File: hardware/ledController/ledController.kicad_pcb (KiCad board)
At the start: 2 copper layers, 50 x 50 mm, 33 parts, among them IC1 PIC16F1769-I_ML, J1 Conn_01x06, J2 Screw_Terminal_01x02, J3 Screw_Terminal_01x02, J4 Conn_01x06, J5 Conn_01x02_Male, M1 LM2596_module, Q1 FMMT458TA, Q2 BUJ302AD

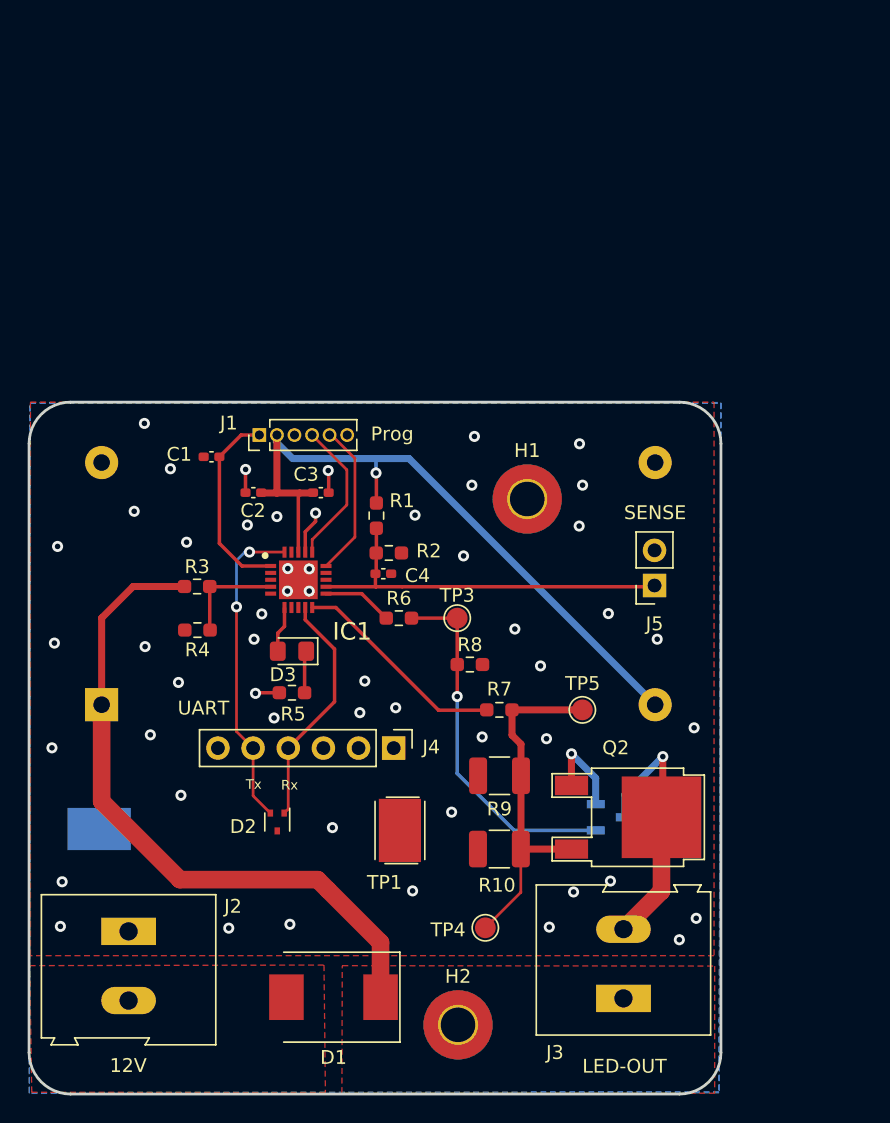
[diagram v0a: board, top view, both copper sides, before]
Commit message: Minor changes
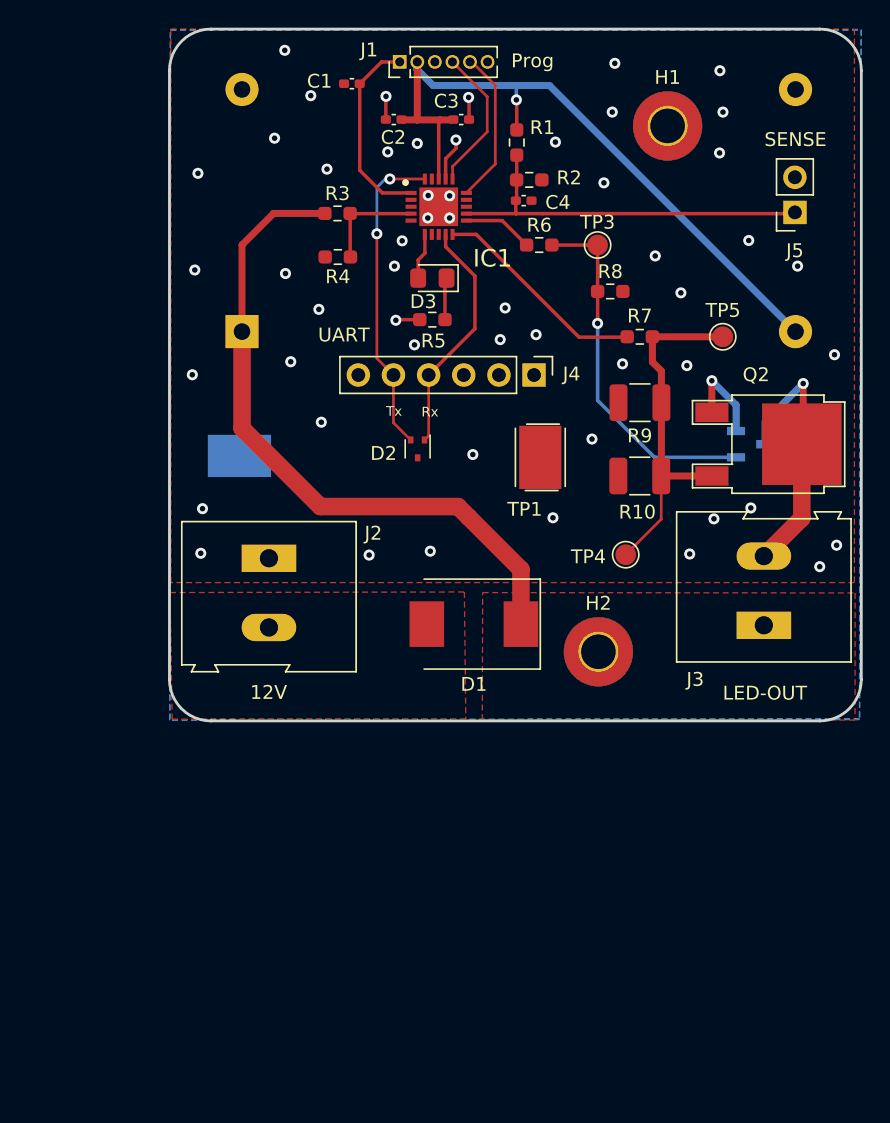
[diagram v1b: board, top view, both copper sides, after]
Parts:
- moved C4 28.8 mm to (140.7, 89.4)
- moved J1 28.8 mm to (131.8, 79.4)
- moved R10 28.8 mm to (149.1, 109.3)
- moved R2 28.8 mm to (141.1, 87.9)
- moved IC1 28.8 mm to (134.6, 89.9)
- moved C2 28.8 mm to (131.4, 83.6)
- moved C3 28.8 mm to (136.2, 83.6)
- moved D1 28.8 mm to (137.1, 120.0)
- moved D2 28.8 mm to (133.1, 107.4)
- moved D3 28.8 mm to (134.1, 95.0)
- moved H1 28.8 mm to (151.1, 84.0)
- moved H2 28.8 mm to (146.1, 122.0)
- moved J4 28.8 mm to (141.5, 102.0)
- moved J5 28.8 mm to (160.3, 90.3)
- moved M1 28.8 mm to (140.4, 90.9)
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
